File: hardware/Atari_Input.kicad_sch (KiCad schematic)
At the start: 11 parts

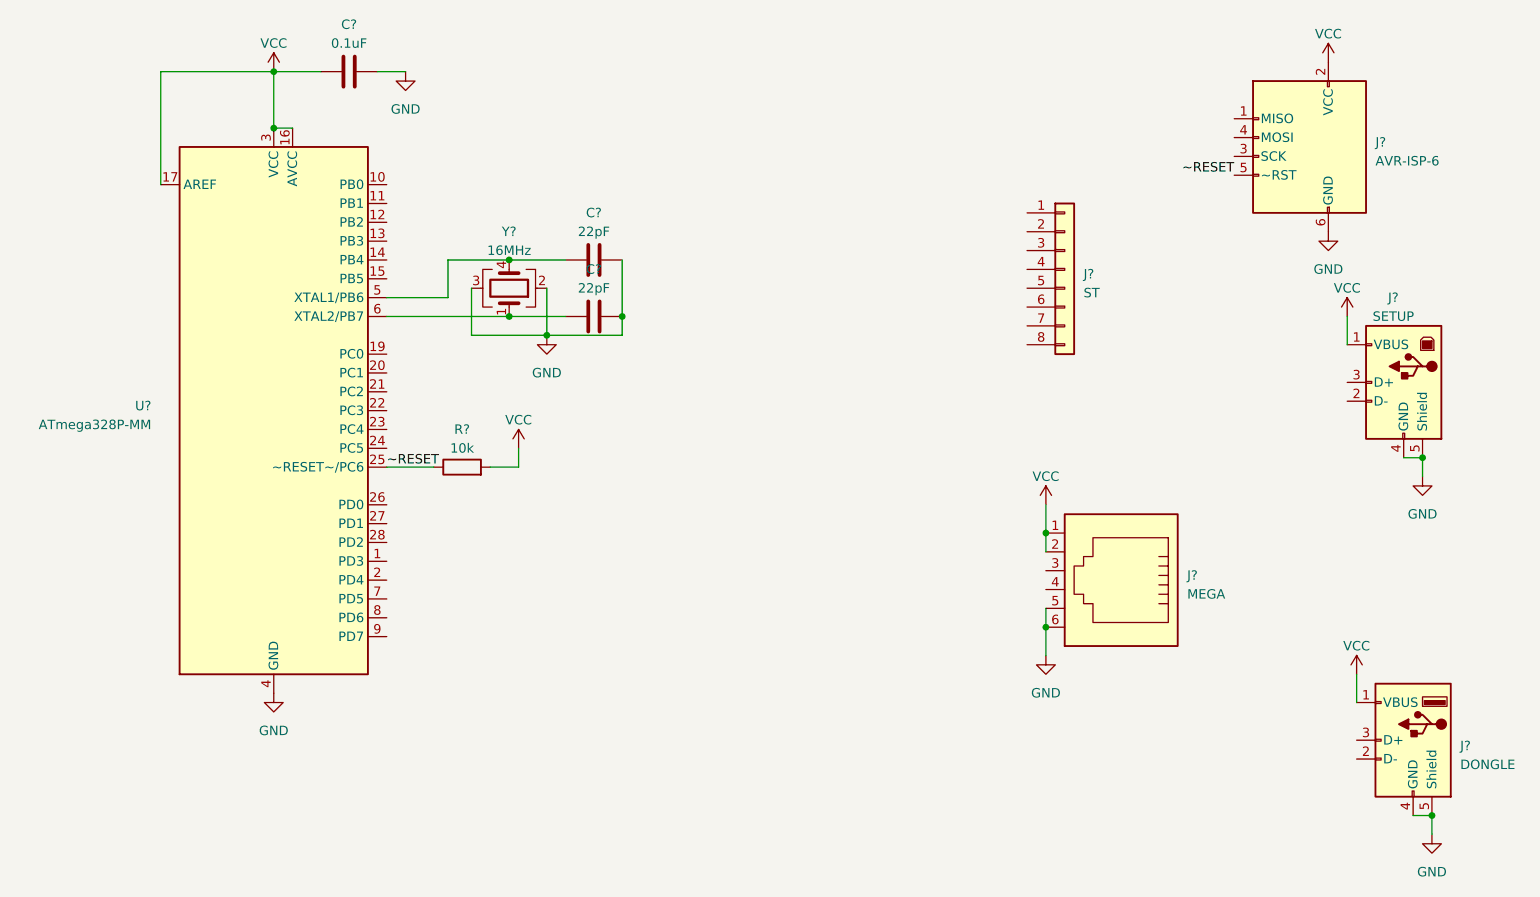
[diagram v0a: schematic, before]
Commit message: bdfijbjkl
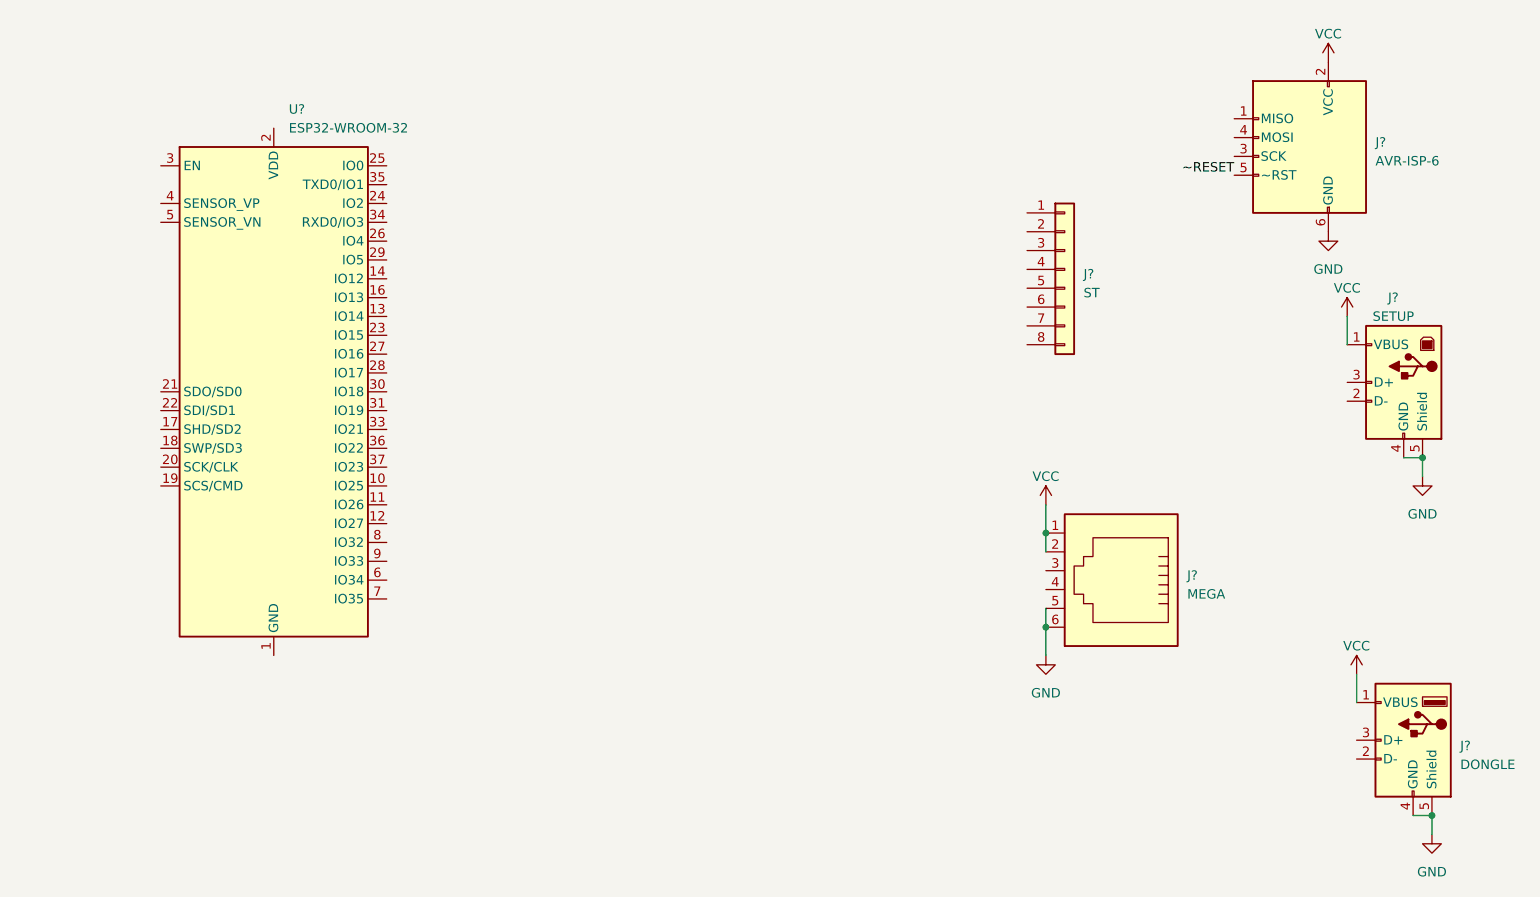
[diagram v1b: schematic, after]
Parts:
- removed C?: 0.1uF, symbol Device:C
- removed C? (x2): 22pF, symbol Device:C
- removed R?: 10k, symbol Device:R
- removed U?: ATmega328P-MM, Package_DFN_QFN:QFN-28-1EP_4x4mm_P0.45mm_EP2.4x2.4mm, symbol MCU_Microchip_ATmega:ATmega328P-MM
- removed Y?: 16MHz, symbol Device:Crystal_GND23
- added U?: ESP32-WROOM-32, RF_Module:ESP32-WROOM-32, symbol RF_Module:ESP32-WROOM-32
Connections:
- new net: U?.1 (GND), U?.15 (GND), U?.38 (GND), U?.39 (GND)
